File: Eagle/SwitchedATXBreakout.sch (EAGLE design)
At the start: 37 parts, among them K1 ALF1P05, K2 ALF1P05, K3 ALF1P05, K4 ALF1P05, K5 ALF1P05, X1 22-23-2091, X2 5566-24

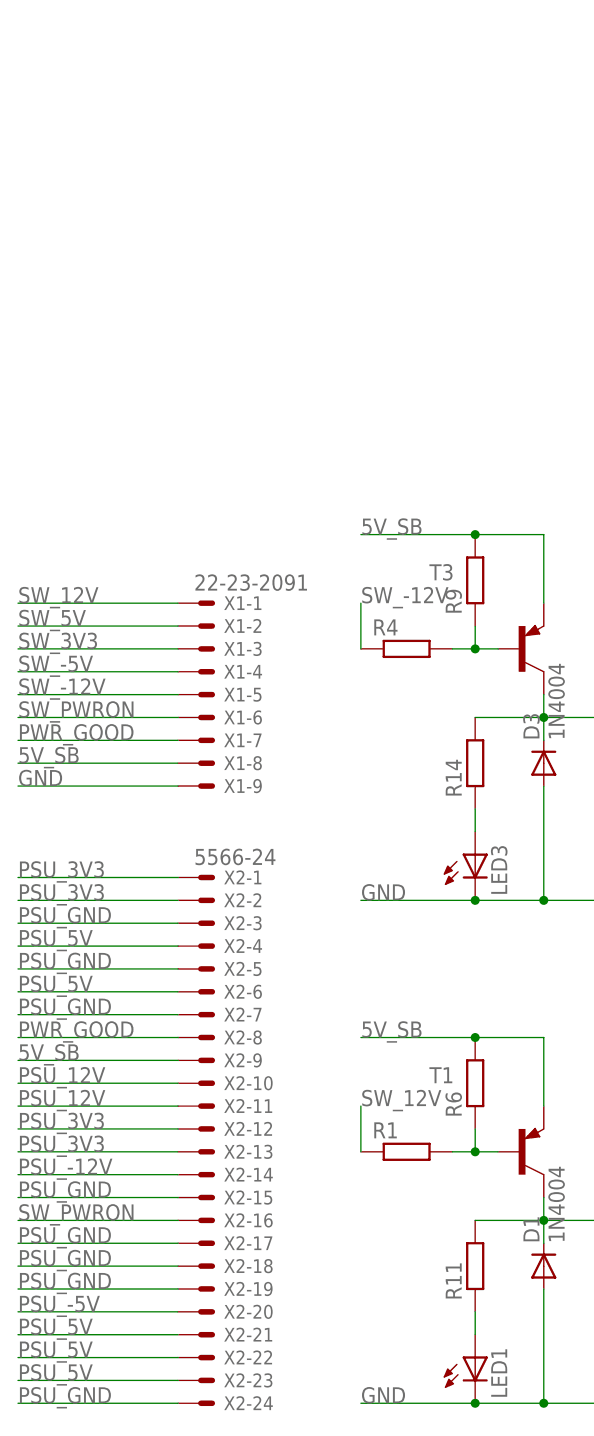
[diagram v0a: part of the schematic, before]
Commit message: More work on board
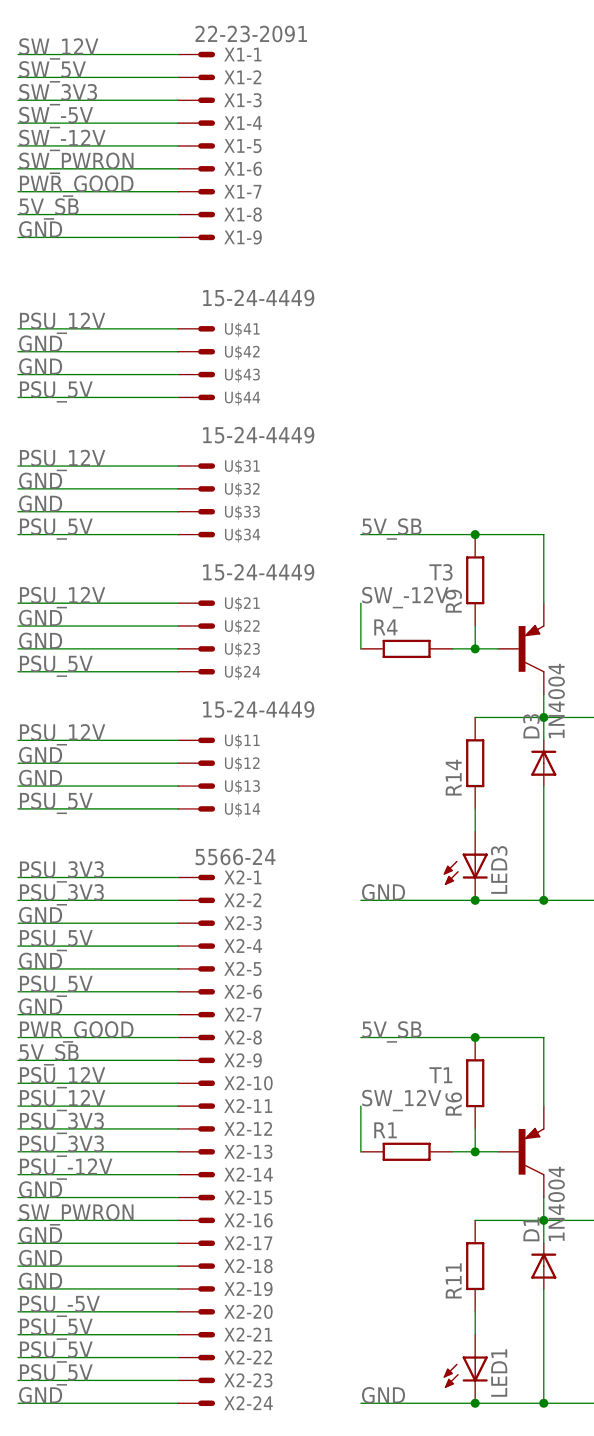
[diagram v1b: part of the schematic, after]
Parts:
- added U$1, U$2, U$3, U$4: 15-24-4449, con-molex-additional:15-24-4449
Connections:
- removed net PSU_GND: X2-15.S, X2-17.S, X2-18.S, X2-19.S, X2-24.S, X2-3.S, X2-5.S, X2-7.S
- net GND: now also U$12.P$1, U$13.P$1, U$22.P$1, U$23.P$1, U$32.P$1, U$33.P$1, U$42.P$1, U$43.P$1, X2-15.S, X2-17.S, X2-18.S, X2-19.S, X2-24.S, X2-3.S, X2-5.S, X2-7.S
- net PSU_12V: now also U$11.P$1, U$21.P$1, U$31.P$1, U$41.P$1
- net PSU_5V: now also U$14.P$1, U$24.P$1, U$34.P$1, U$44.P$1
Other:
- moved on the sheet: X1-1, X1-2, X1-3, X1-4, X1-5, X1-6, X1-7, X1-8, X1-9
